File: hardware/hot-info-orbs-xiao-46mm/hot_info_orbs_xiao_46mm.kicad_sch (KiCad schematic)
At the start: 12 parts, among them SW1 SW_Push, SW2 SW_Push, SW3 SW_Push, U2 XIAO ESP32-S3 Plus

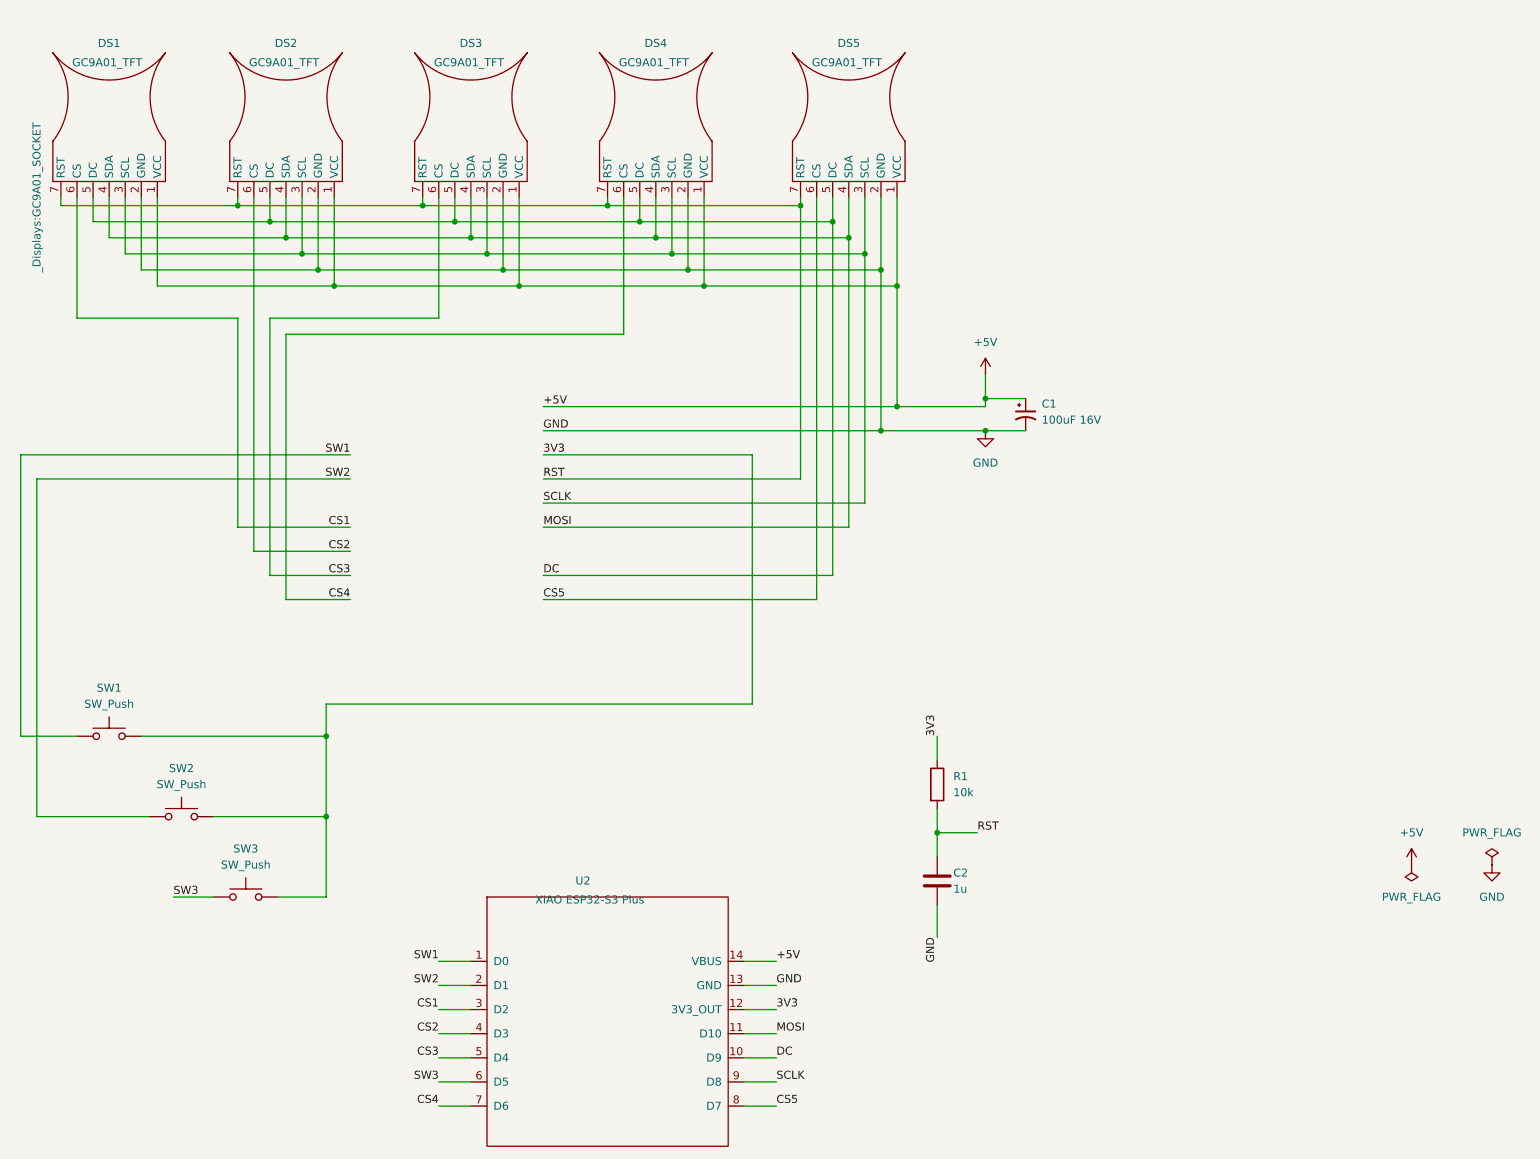
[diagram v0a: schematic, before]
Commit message: 46mm schematic: displays as a labelled block, no wires across the page
Each display pin now has a short stub and its net label, the five displays
sit in a dashed box, and the mid-sheet label column is gone. SW1/SW2 get
labels at the switch like SW3, and the switch bus a 3V3 label. 136 wires,
junctions and labels out, 78 in, by tools/display_block.py; no symbol moved.

Checked against HEAD: kicadxml netlist identical (net names and pins),
ERC 0, DRC 3 known silk warnings / 0 unconnected / 0 parity.

Rejected a hierarchical sheet for the displays: Scott chose a boxed group on
the same page, and a sub-sheet would change every display's symbol path and
need the PCB re-linked. Dropped the +5V/GND labels at C1 too: a label joins
the power net by name, so the netlist is the same without them.

Co-Authored-By: Claude Opus 5.5 <noreply@anthropic.com>
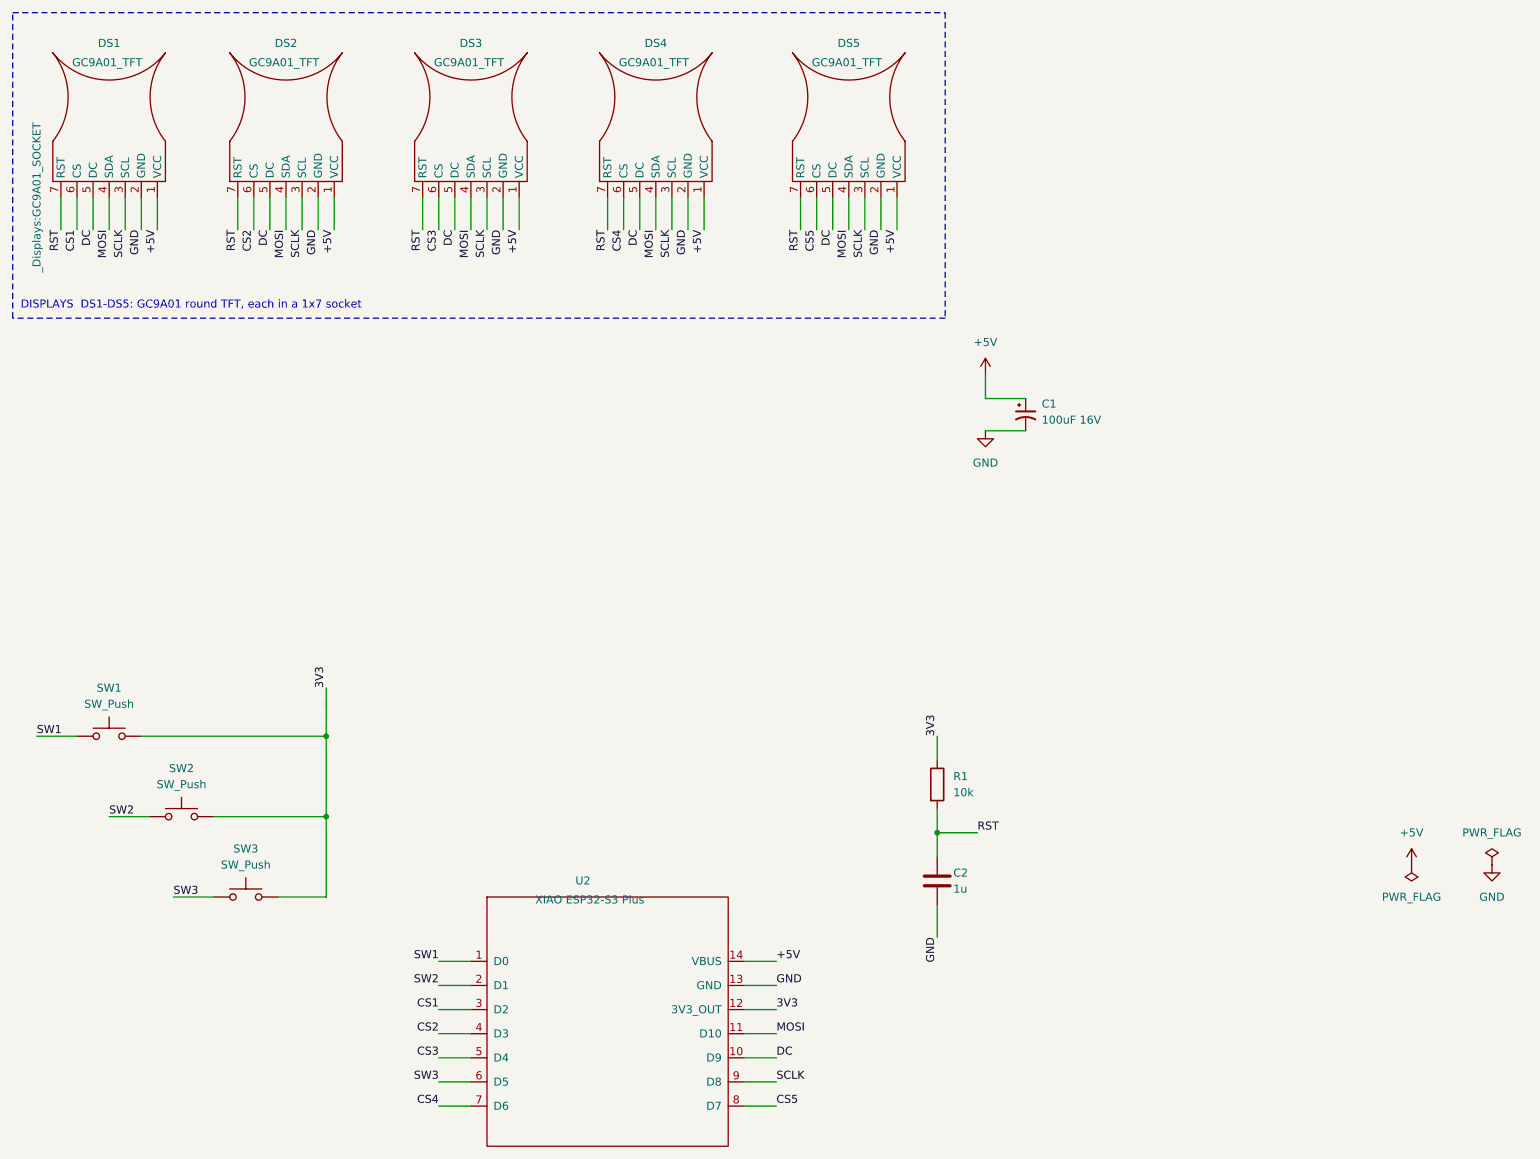
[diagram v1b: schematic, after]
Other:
- note added: "DISPLAYS DS1-DS5: GC9A01 round TFT, each in a 1x7 socket"
